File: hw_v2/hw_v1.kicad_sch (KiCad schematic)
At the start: 53 parts, among them J16 47352-1001, J8 USB_B, J9 Tag connect, SW1 SW_Push, SW2 SW_Push, U13 STM32F407VGTx, U14 TJA1051T-3, U15 25Q16, U16 REF3033, U17 SRV05-4, Y1 32.768kHz, Y2 25MHz

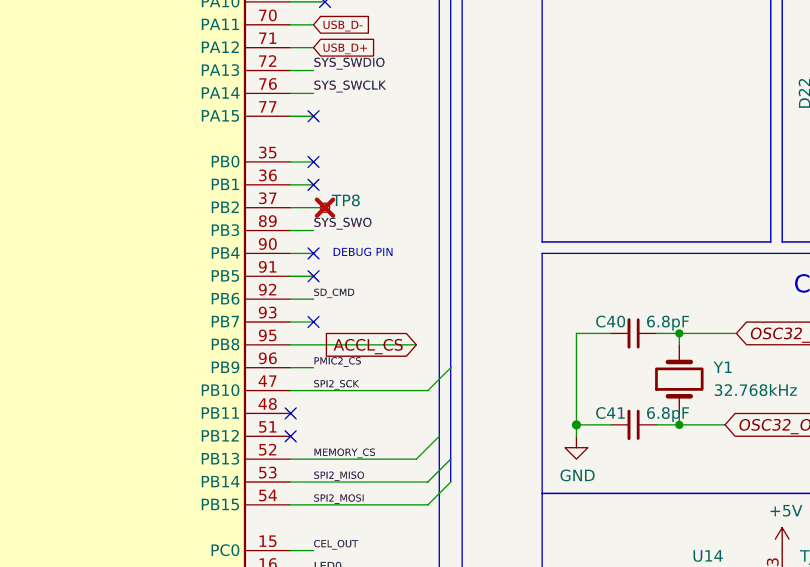
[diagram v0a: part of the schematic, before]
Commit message: wip analog frontend & power
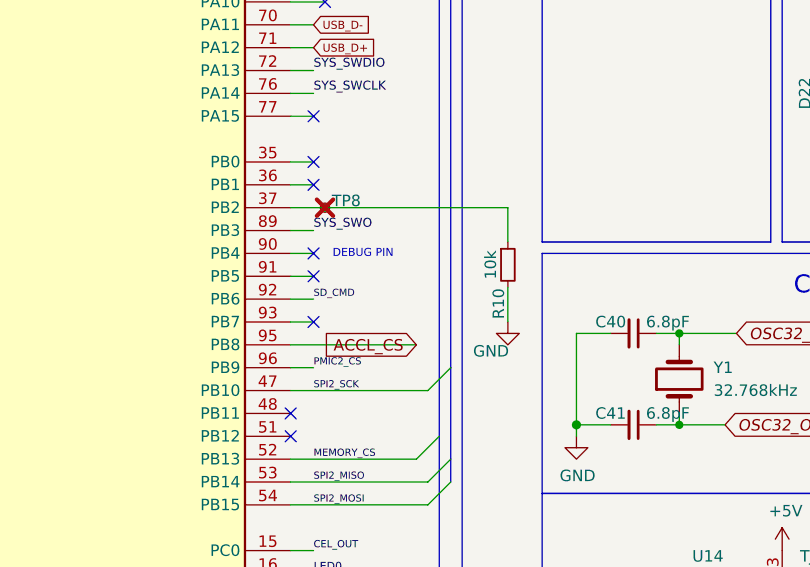
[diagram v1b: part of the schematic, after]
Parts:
- added R10: 10k, Resistor_SMD:R_0603_1608Metric, symbol Device:R_Small
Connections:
- net GND: now also R10.2
- net at TP8.1, U13.37 (PB2): now also R10.1
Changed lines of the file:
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@@
 	)
 	(junction
+		(at 85.09 96.52)
+		(diameter 0)
+		(color 0 0 0 0)
+	)
+	(junction
 		(at 163.83 189.23)
 		(diameter 1.016)
@@
 	(wire
 		(pts
+			(xy 105.41 105.41) (xy 105.41 109.22)
+		)
+		(stroke
+			(width 0)
+			(type default)
+		)
+	)
+	(wire
+		(pts
 			(xy 135.255 43.18) (xy 138.43 43.18)
 		)
@@
 	(wire
 		(pts
+			(xy 85.09 96.52) (xy 105.41 96.52)
+		)
+		(stroke
+			(width 0)
+			(type solid)
+		)
+	)
+	(wire
+		(pts
 			(xy 204.47 87.63) (xy 205.74 87.63)
 		)
@@
 	(wire
 		(pts
-			(xy 85.09 96.52) (xy 81.28 96.52)
+			(xy 81.28 96.52) (xy 85.09 96.52)
 		)
 		(stroke
@@
 	(wire
 		(pts
+			(xy 105.41 100.33) (xy 105.41 96.52)
+		)
+		(stroke
+			(width 0)
+			(type default)
+		)
+	)
+	(wire
+		(pts
 			(xy 144.78 121.92) (xy 144.78 120.65)
 		)
@@
 	(symbol
 		(lib_id "power:GND")
+		(at 105.41 109.22 0)
+		(unit 1)
+		(exclude_from_sim no)
+		(in_bom yes)
+		(on_board yes)
+		(dnp no)
+		(property "Reference" "#PWR053"
+			(at 105.41 115.57 0)
+			(effects
+				(font
+					(size 1.27 1.27)
+				)
+				(hide yes)
+			)
+		)
+		(property "Value" "GND"
+			(at 105.537 112.4712 0)
+			(effects
+				(font
+					(size 1.27 1.27)
+				)
+				(justify right)
+			)
+		)
+		(property "Footprint" ""
+			(at 105.41 109.22 0)
+			(effects
+				(font
+					(size 1.27 1.27)
+				)
+				(hide yes)
+			)
+		)
+		(property "Datasheet" ""
+			(at 105.41 109.22 0)
+			(effects
+				(font
+					(size 1.27 1.27)
+				)
+				(hide yes)
+			)
+		)
+		(property "Description" ""
+			(at 105.41 109.22 0)
+			(effects
+				(font
+					(size 1.27 1.27)
+				)
+				(hide yes)
+			)
+		)
+		(pin "1"
+		)
+		(instances
+			(project "hw_v1"
+				(path "/b3feb07e-be80-40e1-bd13-6cd54c2f8b0c"
+					(reference "#PWR053")
+					(unit 1)
+				)
+			)
+		)
+	)
+	(symbol
+		(lib_id "power:GND")
 		(at 135.89 154.94 0)
 		(unit 1)
@@
 					(unit 1)
 				)
+			)
+		)
+	)
+	(symbol
+		(lib_id "Device:R_Small")
+		(at 105.41 102.87 0)
+		(unit 1)
+		(exclude_from_sim no)
+		(in_bom yes)
+		(on_board yes)
+		(dnp no)
+		(property "Reference" "R10"
+			(at 104.394 107.188 90)
+			(effects
+				(font
+					(size 1.27 1.27)
+				)
+			)
+		)
+		(property "Value" "10k"
+			(at 103.505 102.87 90)
+			(effects
+				(font
+					(size 1.27 1.27)
+				)
+			)
+		)
+		(property "Footprint" "Resistor_SMD:R_0603_1608Metric"
+			(at 105.41 102.87 0)
+			(effects
+				(font
+					(size 1.27 1.27)
+				)
+				(hide yes)
+			)
+		)
+		(property "Datasheet" "~"
+			(at 105.41 102.87 0)
+			(effects
+				(font
+					(size 1.27 1.27)
+				)
+				(hide yes)
+			)
+		)
+		(property "Description" ""
+			(at 105.41 102.87 0)
+			(effects
+				(font
+					(size 1.27 1.27)
+				)
+				(hide yes)
+			)
+		)
+		(property "LCSC" "C115324"
+			(at 105.41 102.87 0)
+			(effects
+				(font
+					(size 1.27 1.27)
+				)
+				(hide yes)
+			)
+		)
+		(property "STOCK" "RES-000118-00"
+			(at 105.41 102.87 0)
+			(effects
+				(font
+					(size 1.27 1.27)
+				)
+				(hide yes)
+			)
+		)
+		(pin "1"
+		)
+		(pin "2"
+		)
+		(instances
+			(project "hw_v1"
+				(path "/b3feb07e-be80-40e1-bd13-6cd54c2f8b0c"
+					(reference "R10")
+					(unit 1)
+				)
